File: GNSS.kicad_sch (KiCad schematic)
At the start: 0 parts

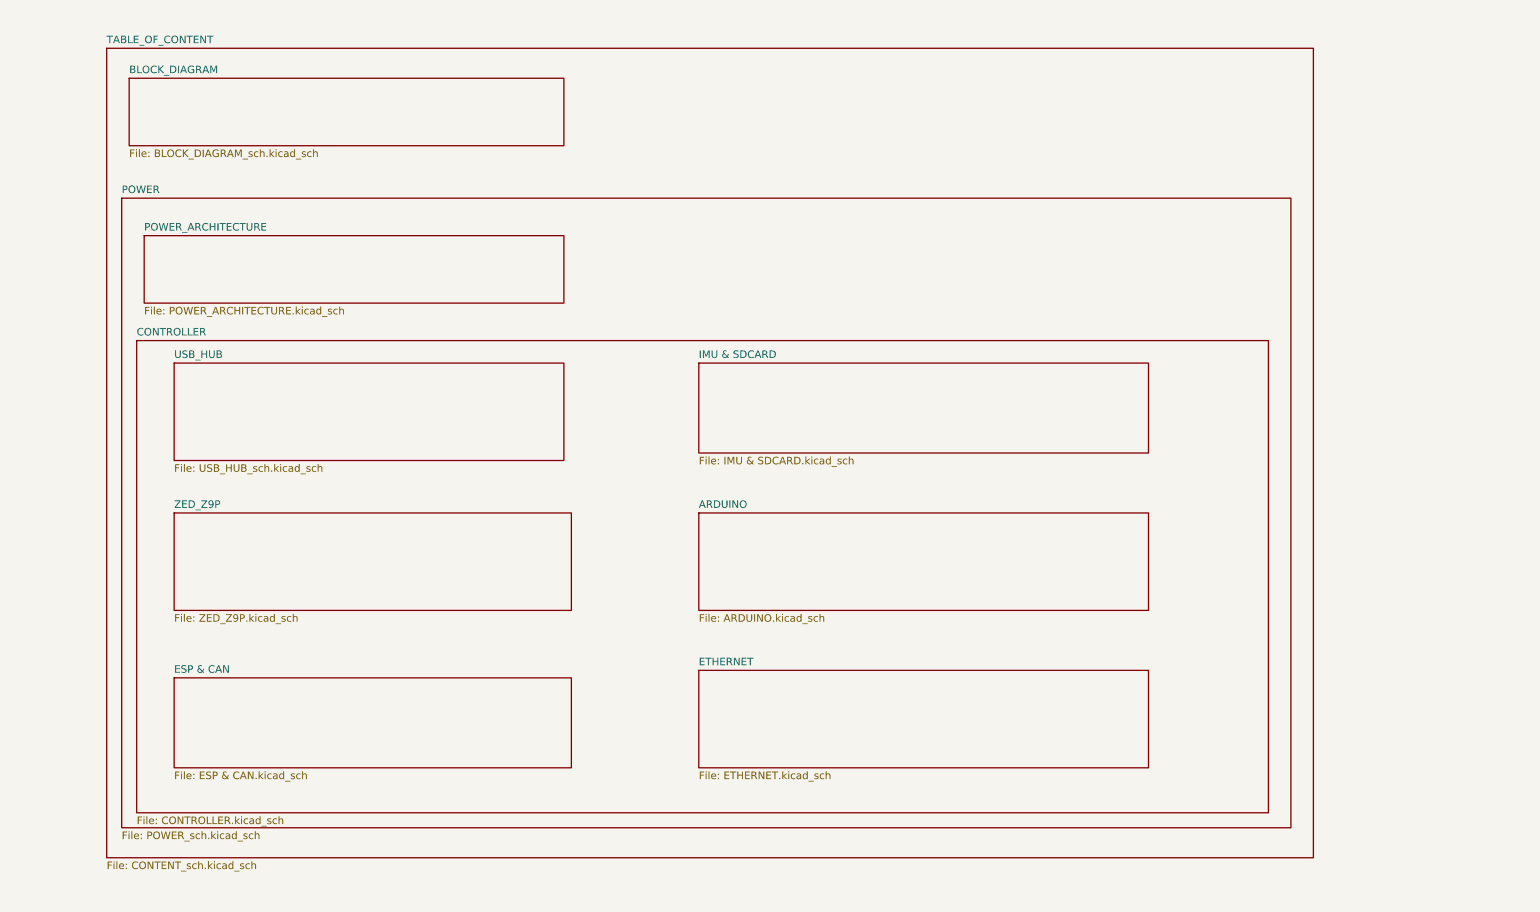
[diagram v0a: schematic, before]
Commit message: full
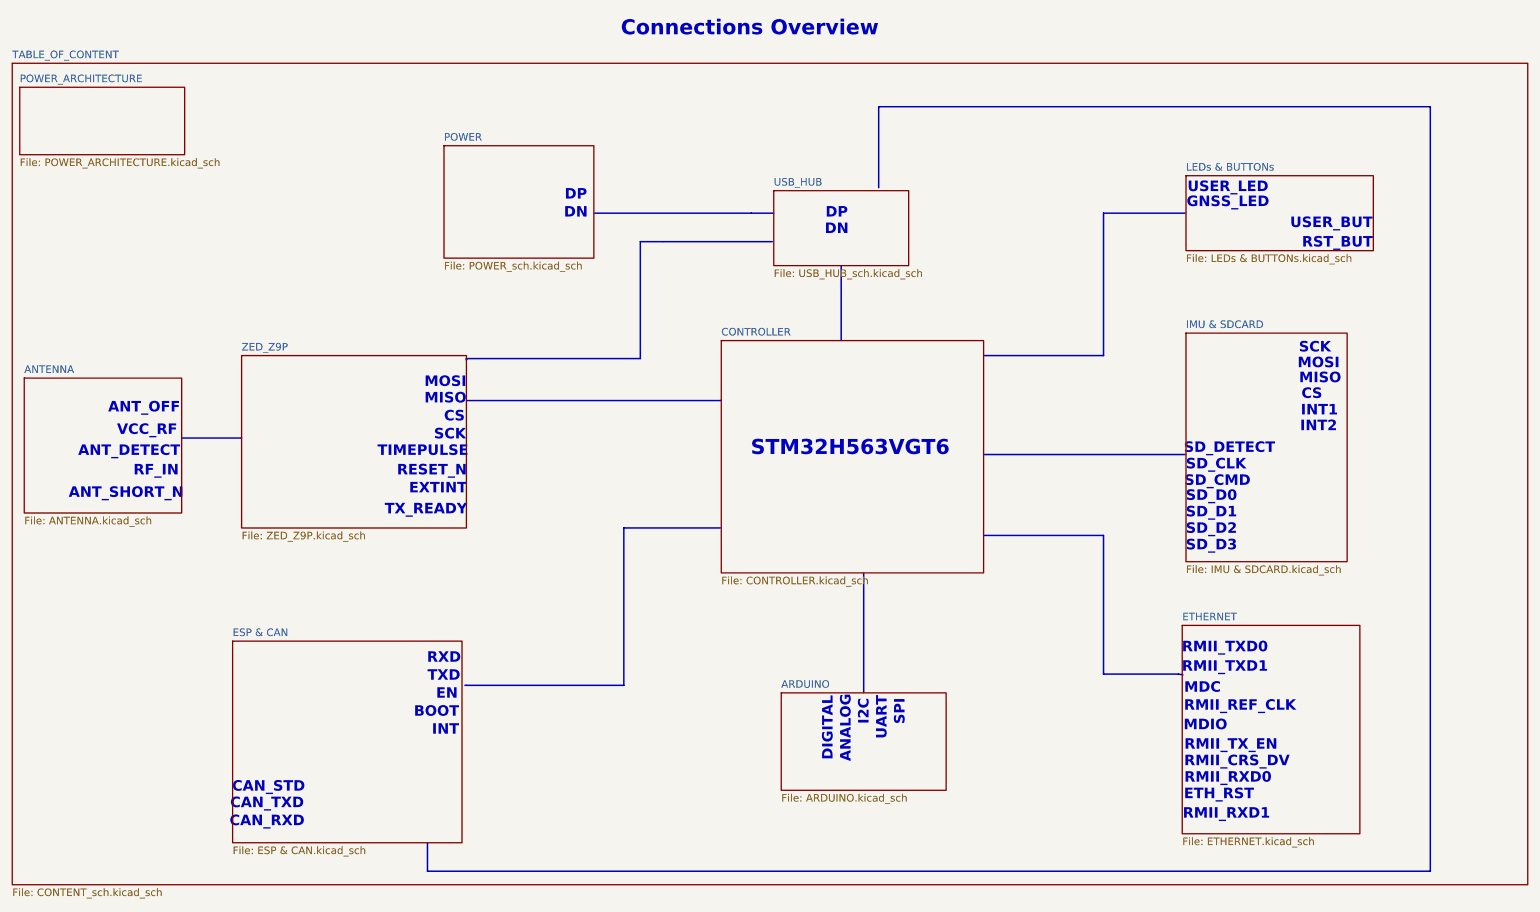
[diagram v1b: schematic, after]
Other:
- removed sheet BLOCK_DIAGRAM
- added sheet ANTENNA (ANTENNA.kicad_sch)
- added sheet LEDs & BUTTONs (LEDs & BUTTONs.kicad_sch)
- note added: "ANALOG"
- note added: "ANT_DETECT"
- note added: "ANT_OFF"
- note added: "ANT_SHORT_N"
- note added: "BOOT"
- note added: "CAN_RXD"
- note added: "CAN_STD"
- note added: "CAN_TXD"
- note added: "CS"
- note added: "Connections Overview"
- note added: "DIGITAL"
- note added: "DN"
- note added: "DP"
- note added: "EN"
- note added: "ETH_RST"
- note added: "EXTINT"
- note added: "GNSS_LED"
- note added: "I2C"
- note added: "INT"
- note added: "INT1"
- note added: "INT2"
- note added: "MDC"
- note added: "MDIO"
- note added: "MISO"
- note added: "MOSI"
- note added: "RESET_N"
- note added: "RF_IN"
- note added: "RMII_CRS_DV"
- note added: "RMII_REF_CLK"
- note added: "RMII_RXD0"
- note added: "RMII_RXD1"
- note added: "RMII_TXD0"
- note added: "RMII_TXD1"
- note added: "RMII_TX_EN"
- note added: "RST_BUT"
- note added: "RXD"
- note added: "SCK"
- note added: "SD_CLK"
- note added: "SD_CMD"
- note added: "SD_D0"
- note added: "SD_D1"
- note added: "SD_D2"
- note added: "SD_D3"
- note added: "SD_DETECT"
- note added: "SPI"
- note added: "STM32H563VGT6"
- note added: "TIMEPULSE"
- note added: "TXD"
- note added: "TX_READY"
- note added: "UART"
- note added: "USER_BUT"
- note added: "USER_LED"
- note added: "VCC_RF"
